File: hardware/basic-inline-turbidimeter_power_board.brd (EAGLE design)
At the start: 12.7 x 45.1 mm, 10 parts, among them IC1 LP298XS

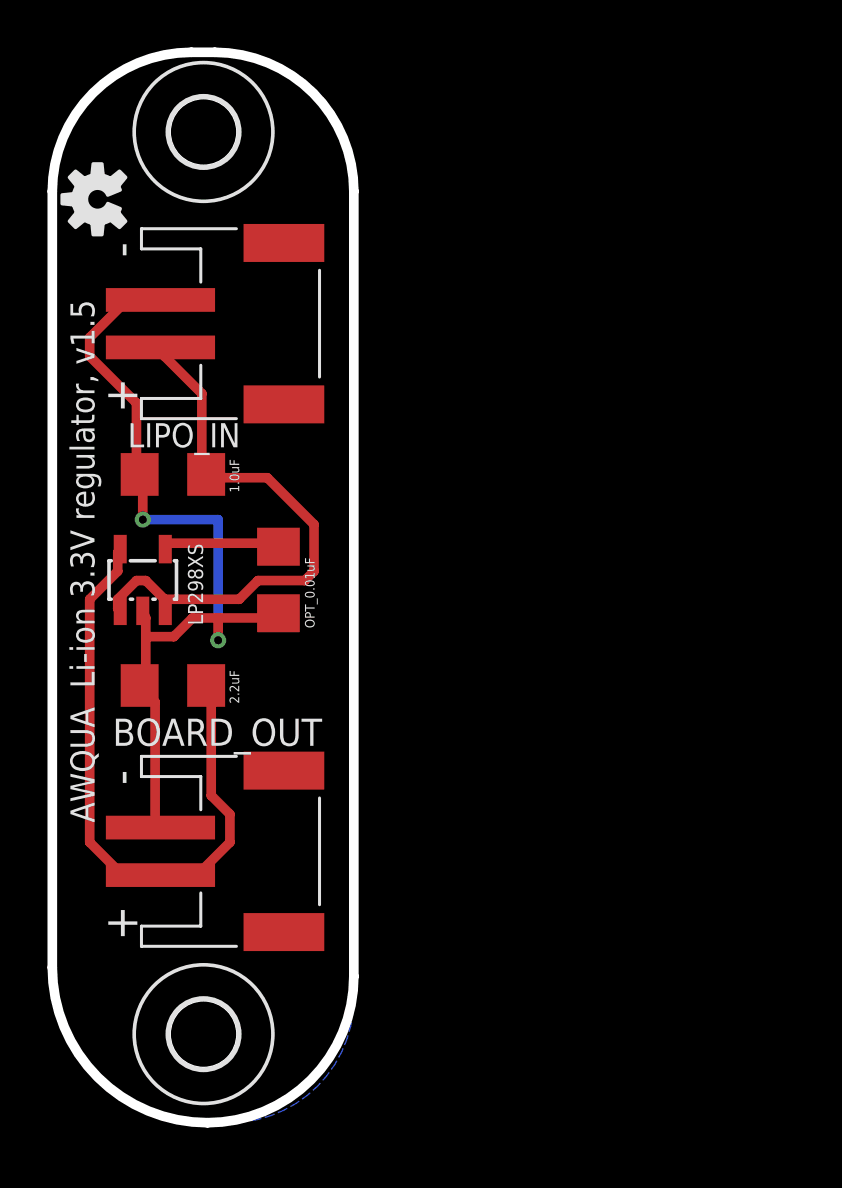
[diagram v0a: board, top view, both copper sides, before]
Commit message: hardware updates
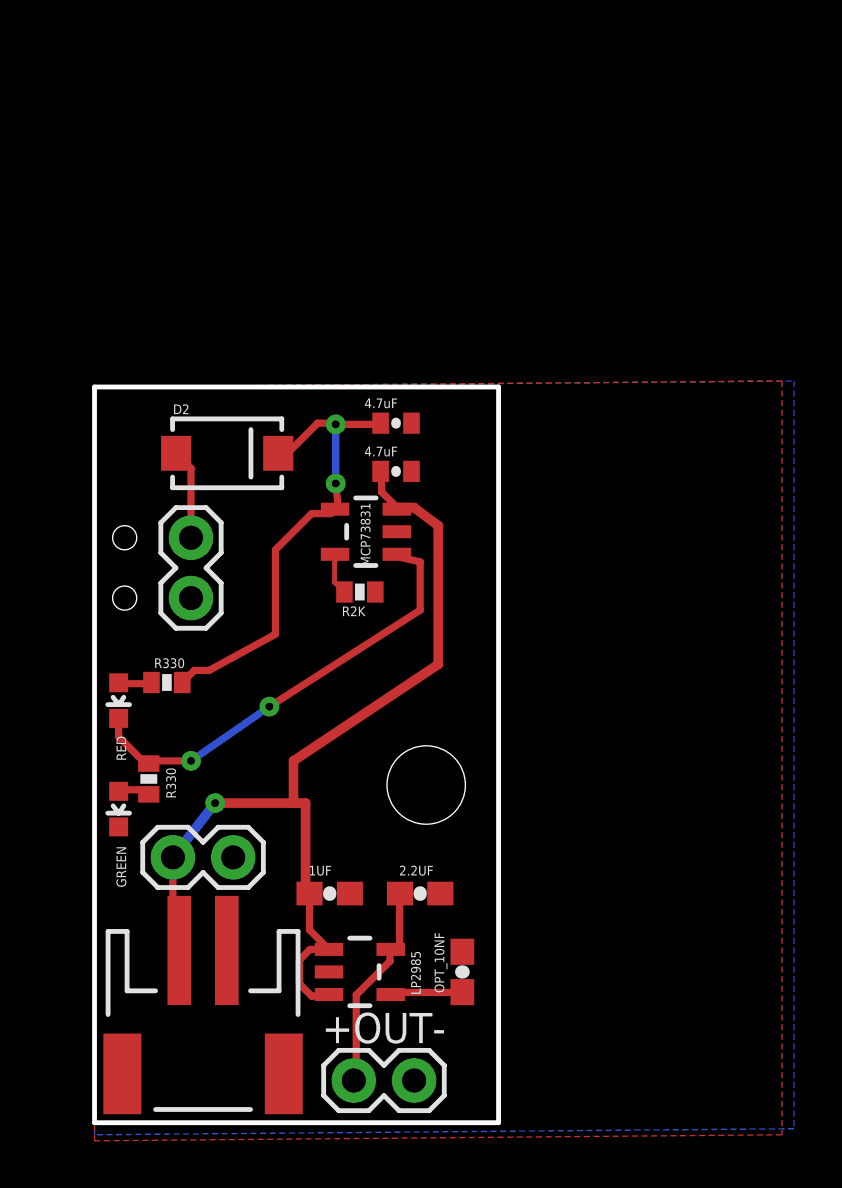
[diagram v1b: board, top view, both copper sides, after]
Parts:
- removed BOARD_OUT, LIPO_IN: (no value), adafruit:JST-PH-2-SMT-RA
- removed C1: OPT_0.01uF, SparkFun-Capacitors:1206
- removed C5: 2.2uF, SparkFun-Capacitors:1206
- removed IC1: LP298XS, adafruit:SOT23-5L
- removed U$1: (no value), SparkFun:OSHW-LOGO-S
- removed U$3, U$5: (no value), holes:2,8
- added +OUT-, JP2: (no value), SparkFun-Connectors:1X02
- added 1UF, 2.2UF, OPT_10NF: (no value), SparkFun-Passives:0603-CAP
- added C4: 4.7uF, SparkFun:0402-CAP
- added D1: GREEN, SparkFun:LED-0603
- added D11: RED, SparkFun:LED-0603
- added D2: MBRA140, SparkFun-DiscreteSemi:SMA-DIODE
- added JMP: (no value), SparkFun:1X02
- added JP1: STAND-OFF, SparkFun:STAND-OFF
- added JP7: LiPo Battery, SparkFun:JST-2-SMD
- added R1: R330, SparkFun:0402-RES
- added R2K: 2K, SparkFun:0402-RES
- added R330: 330, SparkFun:0402-RES
- added U1: MCP73831, SparkFun:SOT23-5
- C3: value 1.0uF -> 4.7uF; device SparkFun-Capacitors:1206 -> SparkFun:0402-CAP
- U$2: value (none) -> LP2985; device SparkFun:OSHW-LOGO-S -> awqua_eagle_library:LP2985
- moved U$2 32.8 mm to (11.7, 7.62), turned to 270 degrees
- moved C3 9.64 mm to (14.5, 29.5), turned to 0 degrees
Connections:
- removed net VOUT: BOARD_OUT.1, C5.1, IC1.5
- new net N$2: D1.A, R1.2
- new net N$3: D11.A, R330.1
- new net N$4: +OUT-.1, 2.2UF.1, U$2.5
- new net N$5: D2.A, JP2.2
- new net PROG: R2K.1, U1.5
- new net STAT: D11.C, R1.1, U1.1
- new net VIN: C3.1, D2.C, R330.2, U1.4
- net GND: now also +OUT-.2, 1UF.2, 2.2UF.2, C4.2, D1.C, JMP.1, JP2.1, JP7.1, OPT_10NF.2, R2K.2, U$2.2, U1.2; no longer BOARD_OUT.2, C1.2, C5.2, IC1.2, LIPO_IN.2
- net N$1: now also OPT_10NF.1, U$2.4; no longer C1.1, IC1.4
- net VCC: now also 1UF.1, C4.1, JMP.2, JP7.2, U$2.1, U$2.3, U1.3; no longer C3.1, IC1.1, IC1.3, LIPO_IN.1
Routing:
- net GND: track 37.2 -> 0.00 mm, vias 2 -> 0
- net VOUT: track 26.9 -> 0.00 mm
- net VIN: track 0.00 -> 19.8 mm, vias 0 -> 2
- net STAT: track 0.00 -> 19.0 mm, vias 0 -> 2
- net VCC: track 24.4 -> 40.4 mm, vias 0 -> 1
- net N$4: track 0.00 -> 8.77 mm
- net N$5: track 0.00 -> 3.82 mm
- net N$1: track 5.14 -> 3.05 mm
- net PROG: track 0.00 -> 1.91 mm
- net N$2: track 0.00 -> 1.49 mm
- net N$3: track 0.00 -> 1.41 mm
- added copper zone on layer 1, net GND
- added copper zone on layer 16, net GND
- removed copper zone on layer 1, net N$2
- removed copper zone on layer 16, net N$3
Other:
- board size 12.7 x 45.1 mm -> 17 x 31 mm
- board text added: "AWQUA power supply v2.1 2016/12/28 github.com/awqua"
- board text removed: "AWQUA Li-ion 3.3V regulator v1.5 2015/08/11 github.com/awqua"
- board text removed: "AWQUA Li-ion 3.3V regulator, v1.5"
